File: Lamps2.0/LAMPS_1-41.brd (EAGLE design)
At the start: 101.6 x 60.3 mm, 83 parts, among them IC2 7805TV, IC4 TLV5618, IC5 TL082P, IC6 TL082P, IC7 7806TV, Q1 STP55NF06L, Q2 STP55NF06L, U1 ARDUINO_MEGA_SHIELD

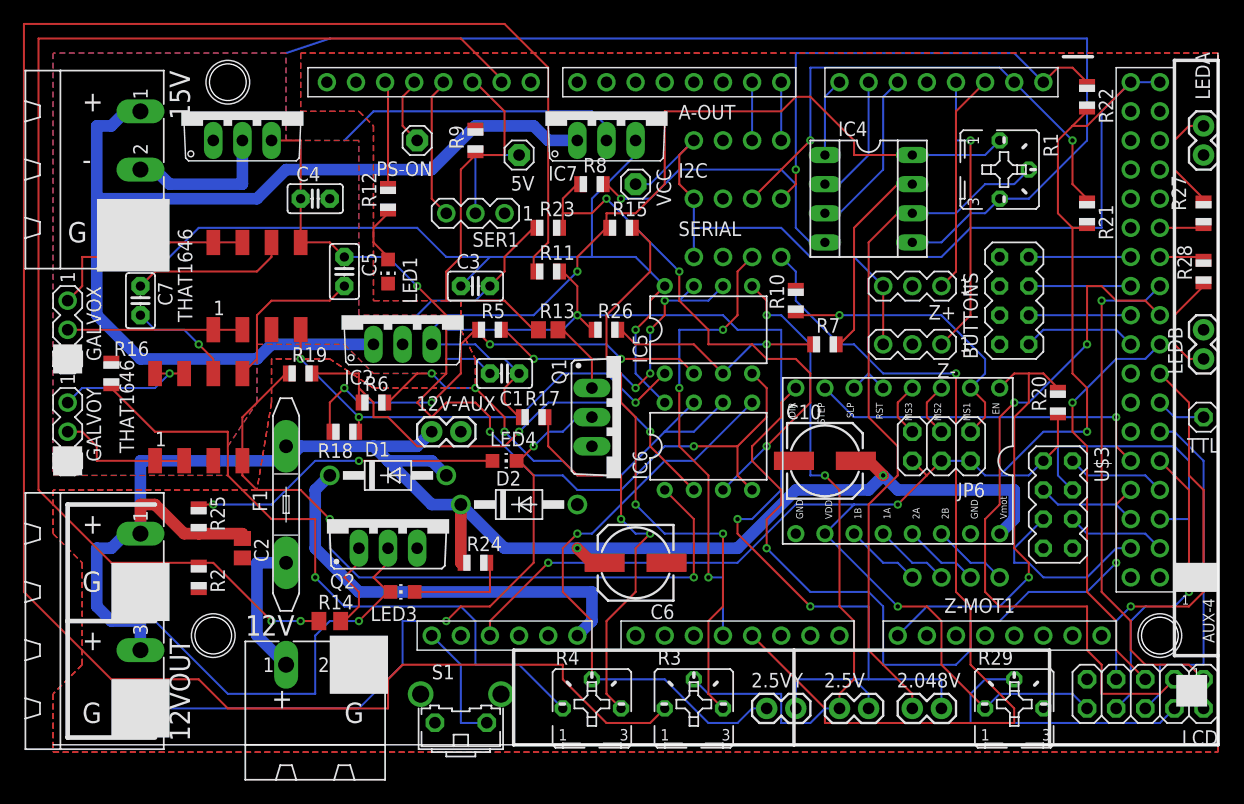
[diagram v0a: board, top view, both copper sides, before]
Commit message: LAMPS 1.0 GERBERS
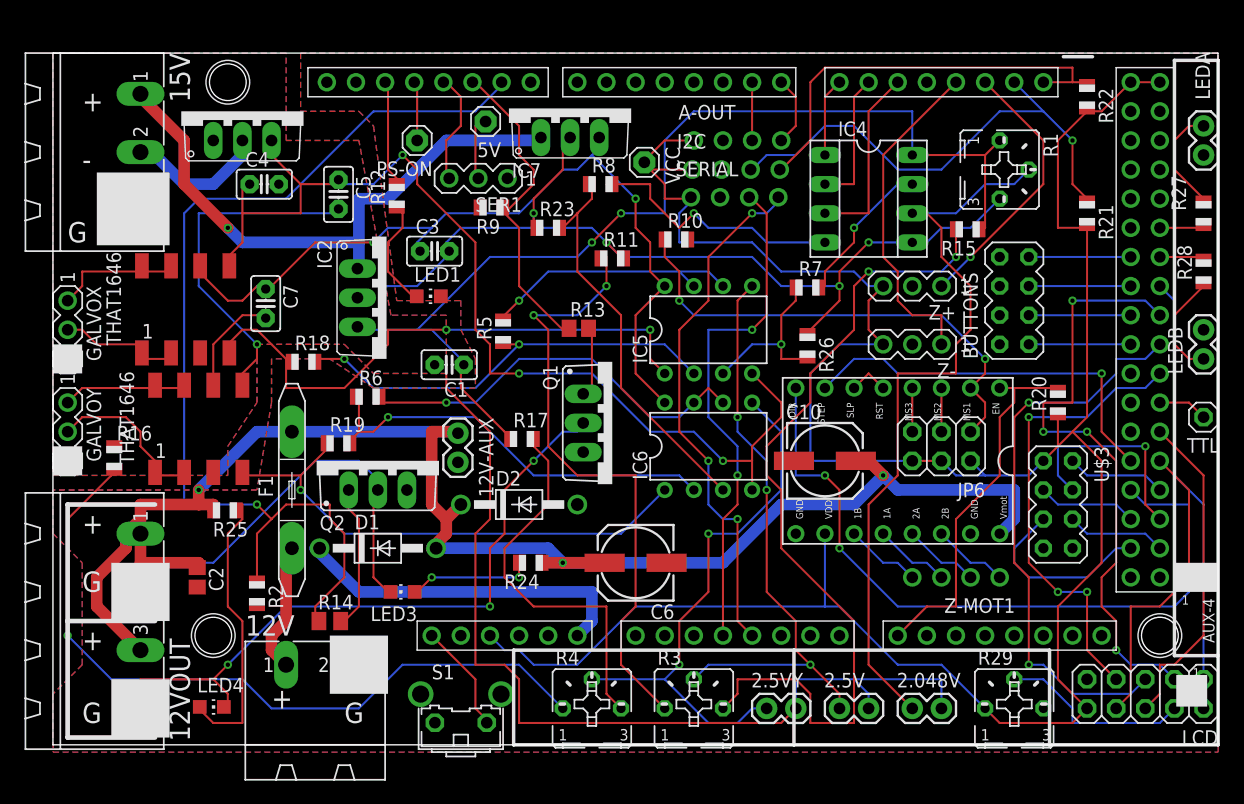
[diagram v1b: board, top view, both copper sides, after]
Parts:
- moved LED4 33.4 mm to (13.8, 11.6)
- moved R15 30.2 mm to (79.8, 53.2), turned to 180 degrees
- moved R26 17.6 mm to (65.8, 43.1), turned to 270 degrees
- moved R10 11.7 mm to (54.4, 52.3), turned to 0 degrees
- moved C7 10.9 mm to (18.5, 46.7)
- moved R16 7.37 mm to (5.33, 33.3)
- moved R18 7.06 mm to (21.8, 41.7), turned to 0 degrees
- moved R19 6.93 mm to (24.9, 34.5)
- moved C5 6.75 mm to (24.9, 56.3)
- moved U$1 6.55 mm to (11.6, 46.2)
- moved D1 6.41 mm to (28.3, 25.4)
- moved R9 6.01 mm to (38.2, 55.1), turned to 180 degrees
- moved R11 5.70 mm to (48.8, 50.7)
- moved R2 5.27 mm to (17.8, 21.5)
- moved SERIAL 5.21 mm to (58.2, 56.0)
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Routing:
- net N$8: track 181.9 -> 53.5 mm, vias 0 -> 2
- net GND_0: track 240.5 -> 163.5 mm, vias 3 -> 4
- net N$2: track 92.1 -> 51.5 mm, vias 0 -> 1
- net A4: track 80.3 -> 46.2 mm, vias 1 -> 3
- net D9: track 111.3 -> 90.1 mm, vias 2 -> 1
- net N$9: track 52.5 -> 73.3 mm
- net POS_6V: track 91.3 -> 72.6 mm, vias 1 -> 2
- net Y_IN: track 64.0 -> 45.5 mm, vias 2 -> 1
- net T2_5: track 14.3 -> 31.0 mm, vias 0 -> 1
- net N$40: track 26.3 -> 42.6 mm, vias 1 -> 2
- net N$22: track 48.9 -> 34.8 mm, vias 3 -> 0
- net D39: track 36.5 -> 49.9 mm, vias 1 -> 2
- net POS_5V: track 81.9 -> 92.7 mm, vias 1 -> 2
- net NEG_6V: track 82.2 -> 92.5 mm
- net D37: track 62.9 -> 53.2 mm, vias 2 -> 4
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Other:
- outline, holes or cut-outs redrawn
